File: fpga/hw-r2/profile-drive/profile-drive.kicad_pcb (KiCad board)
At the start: 4 copper layers, 100 x 50 mm, 110 parts, among them J1 USB-C 16p, J2 DB-25F right-angle, J3 microSD MEM2075, J4 JTAG 1x6, J5 console UART 1x3, J6 flash service 1x7, J7 PROGRAMN button header (optio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, SW1 PROGRAMN button, U1 LFE5U-12F-6TG144C, U2 74LVC245A DATA, U3 74LVC245A CTRL-IN, U4 W25Q128JVSIQ, U5 TLV62568DBV 1V1, U6 TLV62568DBV 3V3, U7 TLV73325PDBV 2V5, X1 25MHz XO 2520 3V3

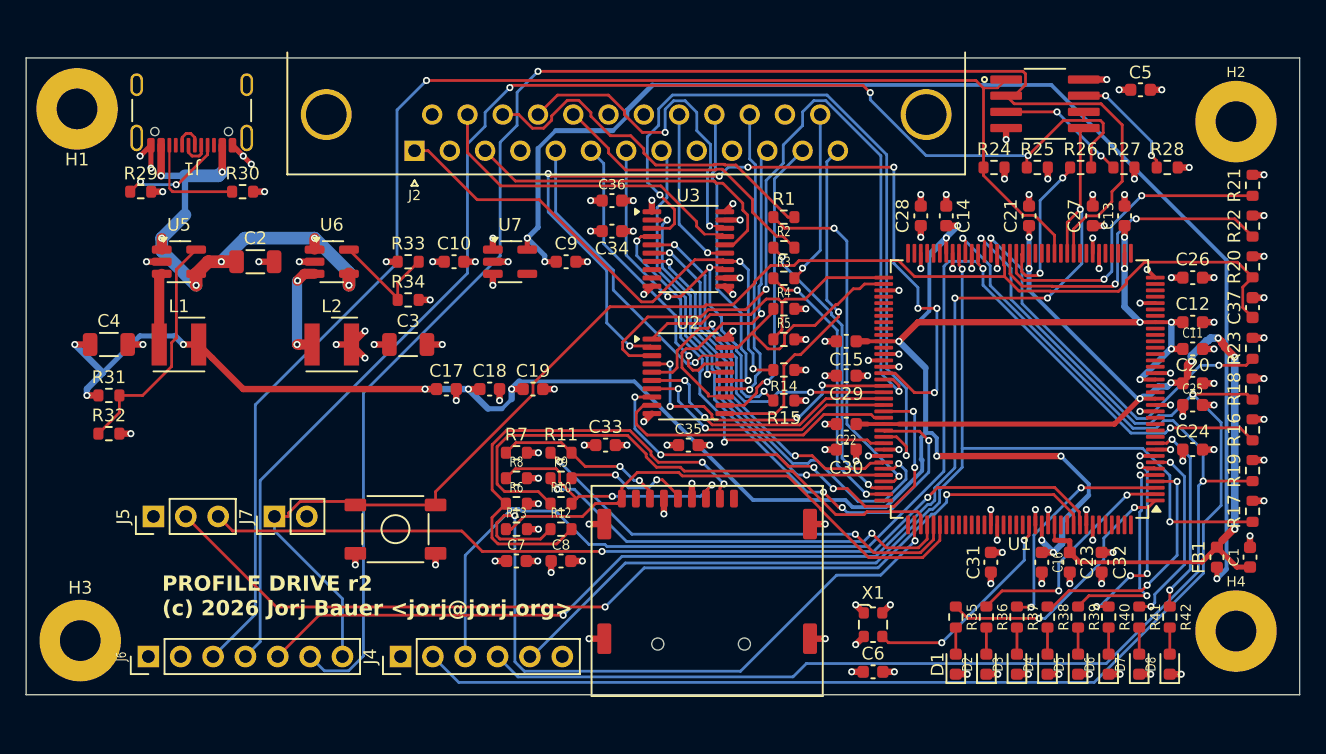
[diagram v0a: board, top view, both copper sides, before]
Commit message: fixups, tweaking
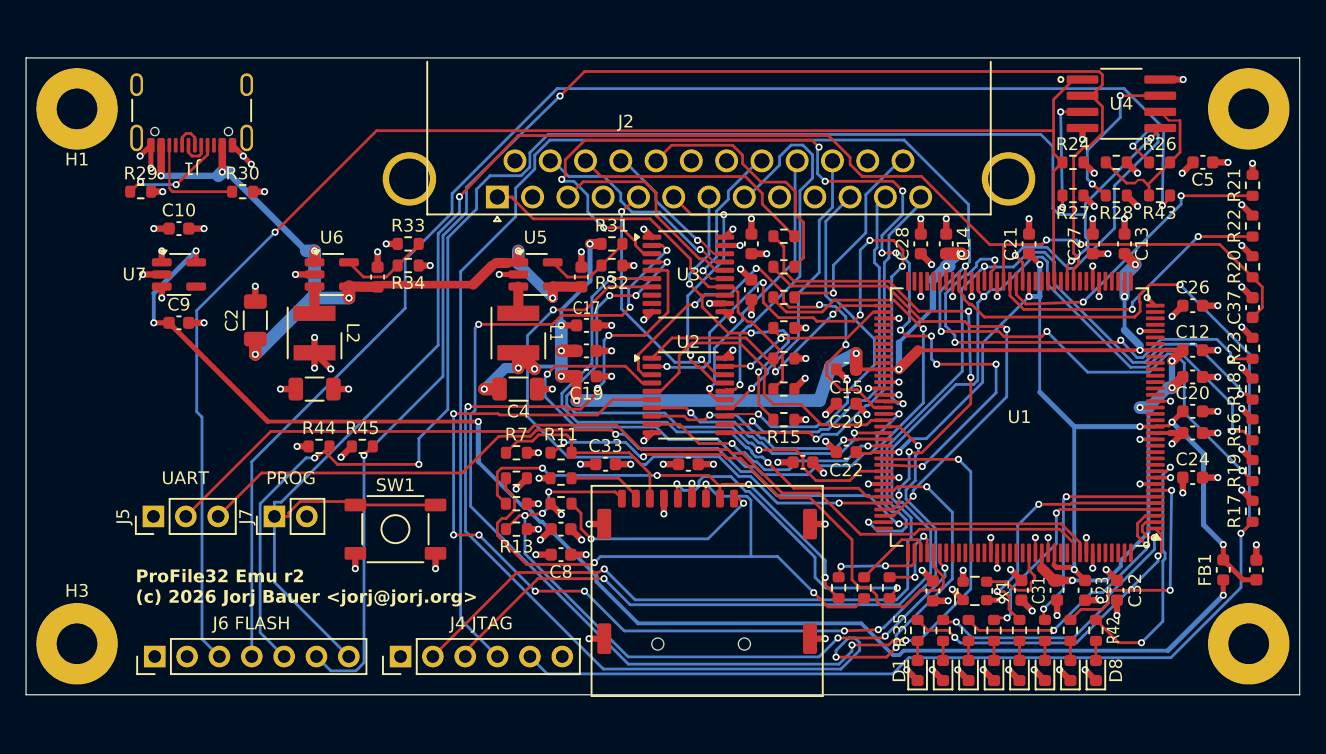
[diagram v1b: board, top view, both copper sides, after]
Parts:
- added C38: 10u, Capacitor_SMD:C_0603_1608Metric, F.Cu at (142.1, 97.2)
- added C39: 10u, Capacitor_SMD:C_0603_1608Metric, F.Cu at (126.1, 97.2)
- added R43: 100R, Resistor_SMD:R_0603_1608Metric, F.Cu at (187.5, 90.8)
- added R44: 10k, Resistor_SMD:R_0603_1608Metric, F.Cu at (121.5, 110.5)
- added R45: 10k, Resistor_SMD:R_0603_1608Metric, F.Cu at (124.9, 110.5)
- added R46: 10k, Resistor_SMD:R_0603_1608Metric, F.Cu at (140.5, 113.0)
- added R47: 10k, Resistor_SMD:R_0603_1608Metric, F.Cu at (140.5, 115.0)
- J2: value DB-25F right-angle -> NorComp 182-025-213R561; footprint Connector_Dsub:DSUB-25_Socket_Horizontal_P2.77x2.84mm_EdgePinOffset4.94mm_Housed_MountingHolesOffset4.94mm -> device:DSUB-25_Female_Horizontal_NorComp_182-025-213R561
- moved R32 41.6 mm to (144.5, 96.3)
- moved R31 41.3 mm to (144.5, 94.6)
- moved C4 32.3 mm to (137.2, 106.0)
- moved C9 30.8 mm to (110.5, 100.8)
- moved U5 28.0 mm to (138.5, 97.0)
- moved R9 27.2 mm to (166.3, 121.6), turned to -90 degrees
- moved L1 26.7 mm to (137.2, 101.6), turned to -90 degrees
- moved U7 26.0 mm to (110.5, 97.0)
- moved R10 24.7 mm to (164.3, 121.6), turned to -90 degrees
- moved R12 22.3 mm to (162.3, 121.6), turned to -90 degrees
- moved C10 21.8 mm to (110.5, 93.4)
- moved C17 12.1 mm to (142.5, 101.0)
- moved C34 11.9 mm to (155.4, 98.2), turned to 90 degrees
- moved C36 11.5 mm to (155.4, 94.6), turned to 90 degrees
- moved X1 8.43 mm to (173.0, 121.8), turned to 90 degrees
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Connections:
- J3 pad 1: unconnected-(J3-DAT2-Pad1) -> /SD card/SD_DAT2
- J3 pad 8: unconnected-(J3-DAT1-Pad8) -> /SD card/SD_DAT1
- J6 pad 4: /Configuration/SPI_CLK_R -> /Configuration/SPI_CLK_J6
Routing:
- net /Configuration/SPI_CLK_J6: track 0.00 -> 110.7 mm, vias 0 -> 1
- net /Configuration/SPI_CLK_R: track 109.3 -> 13.0 mm, vias 3 -> 0
- net Net-(U1C-FPGA_PRES_N): track 30.0 -> 98.8 mm, vias 2 -> 6
- net Net-(U1C-FPGA_PD4): track 21.3 -> 83.6 mm, vias 2 -> 8
- net Net-(U1C-FPGA_PCMD_N): track 45.3 -> 97.7 mm, vias 4 -> 6
- net Net-(U1D-FPGA_SD_CS_N): track 56.0 -> 7.84 mm
- net +1V1: track 177.5 -> 133.4 mm
- net Net-(U1D-FPGA_SD_MOSI): track 45.1 -> 6.54 mm
- net Net-(U1D-FPGA_SD_CLK): track 34.0 -> 6.92 mm
- net /SD card/SD_MOSI: track 20.2 -> 47.1 mm, vias 2 -> 3
- net /Configuration/PROGRAMN: track 108.1 -> 134.7 mm, vias 0 -> 3
- net Net-(U1C-FPGA_PD1): track 60.4 -> 34.6 mm, vias 2 -> 4
- net /Configuration/SPI_MOSI: track 99.0 -> 122.9 mm
- net JTAG_TCK: track 101.1 -> 125.0 mm, vias 2 -> 4
- net Net-(U1C-FPGA_PD0): track 70.2 -> 46.6 mm, vias 8 -> 6
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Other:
- board text added: "J4 JTAG"
- board text added: "J6 FLASH"
- board text added: "PROG"
- board text added: "ProFile32 Emu r2 (c) 2026 Jorj Bauer <jorj@jorj.org>"
- board text added: "UART"
- board text removed: "PROFILE DRIVE r2 (c) 2026 Jorj Bauer <jorj@jorj.org>"

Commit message: more fixes, and r2 gerber first pass
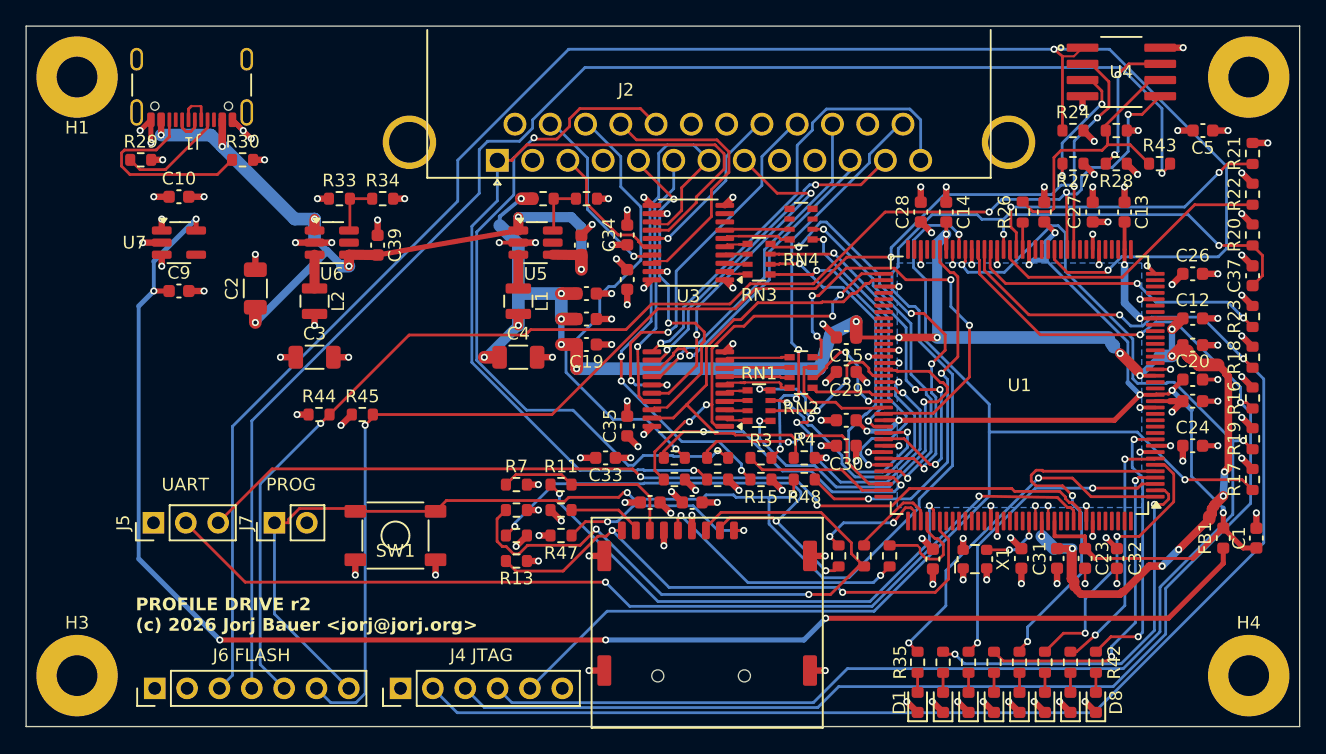
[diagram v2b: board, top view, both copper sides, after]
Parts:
- added R48: 100R, Resistor_SMD:R_0603_1608Metric, F.Cu at (159.6, 113.1)
- added RN1: 47R, Resistor_SMD:R_Array_Convex_4x0603, F.Cu at (156.1, 107.3)
- added RN2: 47R, Resistor_SMD:R_Array_Convex_4x0603, F.Cu at (159.3, 104.7)
- added RN3: 47R, Resistor_SMD:R_Array_Convex_4x0603, F.Cu at (156.1, 95.8)
- added RN4: 47R, Resistor_SMD:R_Array_Convex_4x0603, F.Cu at (159.3, 93.0)
- L1, L2: value 2u2 -> 1u0; footprint Inductor_SMD_Wurth:L_Wurth_WE-LQSH-4020 -> device:L_Murata_DFE252012F
- R31: value 100k -> 84.5k
- R32: value 120k -> 100k
- U5: value TLV62568DBV 1V1 -> TPS62A01A 1V1; footprint Package_TO_SOT_SMD:SOT-23-5_HandSoldering -> Package_TO_SOT_SMD:SOT-23-6_Handsoldering
- U6: value TLV62568DBV 3V3 -> TPS62A01A 3V3; footprint Package_TO_SOT_SMD:SOT-23-5_HandSoldering -> Package_TO_SOT_SMD:SOT-23-6_Handsoldering
- moved R1 19.4 mm to (149.4, 111.4)
- moved R2 15.9 mm to (152.8, 111.4)
- moved R5 12.8 mm to (149.4, 113.1)
- moved R3 12.7 mm to (156.2, 111.4)
- moved R26 11.4 mm to (176.8, 92.1), turned to 90 degrees
- moved C8 11.1 mm to (150.8, 114.9)
- moved C34 10.7 mm to (145.7, 93.9)
- moved R4 10.3 mm to (159.6, 111.4)
- moved C36 10.1 mm to (145.7, 97.4)
- moved R14 8.80 mm to (152.8, 113.1)
- moved C7 7.31 mm to (147.5, 114.9)
- moved R31 6.46 mm to (139.1, 91.0)
- moved R33 6.46 mm to (123.1, 91.0)
- moved C35 5.66 mm to (145.7, 108.9), turned to 90 degrees
- moved R32 5.62 mm to (142.5, 91.0)
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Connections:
- U1 pad 67: unconnected-(U1G-IO-Pad67) -> FPGA_REBOOT
- U2 pad 2: Net-(U1C-FPGA_PD0) -> Net-(U2-A1)
- U2 pad 3: Net-(U1C-FPGA_PD1) -> Net-(U2-A2)
- U2 pad 4: Net-(U1C-FPGA_PD2) -> Net-(U2-A3)
- U2 pad 5: Net-(U1C-FPGA_PD3) -> Net-(U2-A4)
- U2 pad 6: Net-(U1C-FPGA_PD4) -> Net-(U2-A5)
- U2 pad 7: Net-(U1C-FPGA_PD5) -> Net-(U2-A6)
- U2 pad 8: Net-(U1C-FPGA_PD6) -> Net-(U2-A7)
- U2 pad 9: Net-(U1C-FPGA_PD7) -> Net-(U2-A8)
- U3 pad 2: Net-(U1C-FPGA_PCMD_N) -> Net-(U3-A1)
- U3 pad 3: Net-(U1C-FPGA_PSTRB_N) -> Net-(U3-A2)
- U3 pad 4: Net-(U1C-FPGA_PRW) -> Net-(U3-A3)
- U3 pad 5: Net-(U1C-FPGA_PRES_N) -> Net-(U3-A4)
- U3 pad 6: Net-(U1C-FPGA_PH0) -> Net-(U3-A5)
- U3 pad 7: Net-(U1C-FPGA_AUX7) -> Net-(U3-A6)
- U5 pad 5: /Power/FB_1V1 -> unconnected-(U5-PG-Pad5)
- U6 pad 5: /Power/FB_3V3 -> unconnected-(U6-PG-Pad5)
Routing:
- net Net-(U1C-FPGA_PD4): track 83.6 -> 5.82 mm, vias 8 -> 0
- net Net-(U1C-FPGA_PCMD_N): track 97.7 -> 20.2 mm, vias 6 -> 2
- net Net-(U1C-FPGA_PRES_N): track 98.8 -> 34.1 mm, vias 6 -> 4
- net Net-(U1C-FPGA_PSTRB_N): track 79.2 -> 31.2 mm, vias 12 -> 2
- net /ProFile bus/PPARITY: track 19.8 -> 54.9 mm, vias 0 -> 2
- net /ProFile bus/PH0: track 32.0 -> 66.8 mm, vias 0 -> 1
- net FPGA_REBOOT: track 0.00 -> 30.4 mm, vias 0 -> 2
- net /Configuration/SPI_CS_N: track 118.8 -> 147.6 mm, vias 1 -> 2
- net Net-(U1C-FPGA_PCHK): track 36.2 -> 11.5 mm, vias 2 -> 0
- net Net-(U1B-MCLK/CCLK): track 25.5 -> 2.11 mm, vias 2 -> 0
- net Net-(U1C-FPGA_PD1): track 34.6 -> 11.7 mm, vias 4 -> 2
- net Net-(U1C-FPGA_PD2): track 44.9 -> 22.7 mm
- net Net-(U1C-FPGA_AUX7): track 49.0 -> 26.8 mm
- net Net-(U1C-FPGA_PPAR): track 39.5 -> 17.5 mm
- net /ProFile bus/XCVR_OE_N: track 15.7 -> 35.6 mm, vias 2 -> 0
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- added copper zone on B.Cu, net +1V1
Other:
- board size 100 x 50 mm -> 100 x 55 mm
- board text added: "PROFILE DRIVE r2 (c) 2026 Jorj Bauer <jorj@jorj.org>"
- board text removed: "ProFile32 Emu r2 (c) 2026 Jorj Bauer <jorj@jorj.org>"
